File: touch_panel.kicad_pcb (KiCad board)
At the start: 2 copper layers, 50.5 x 50.5 mm, 52 parts, among them J1 2x4 SMD 2.0 MM, J2 2x4 Regular, Q1 MMBT2222, Q2 MMBT2222, Q3 MMBT2222, Q4 MMBT2222, Q5 MMBT2222, Q6 MMBT2222, SW1 Reset Switch, U1 TTP223_1, U2 TTP223_2, U3 TTP223_3, U4 ESP-12E

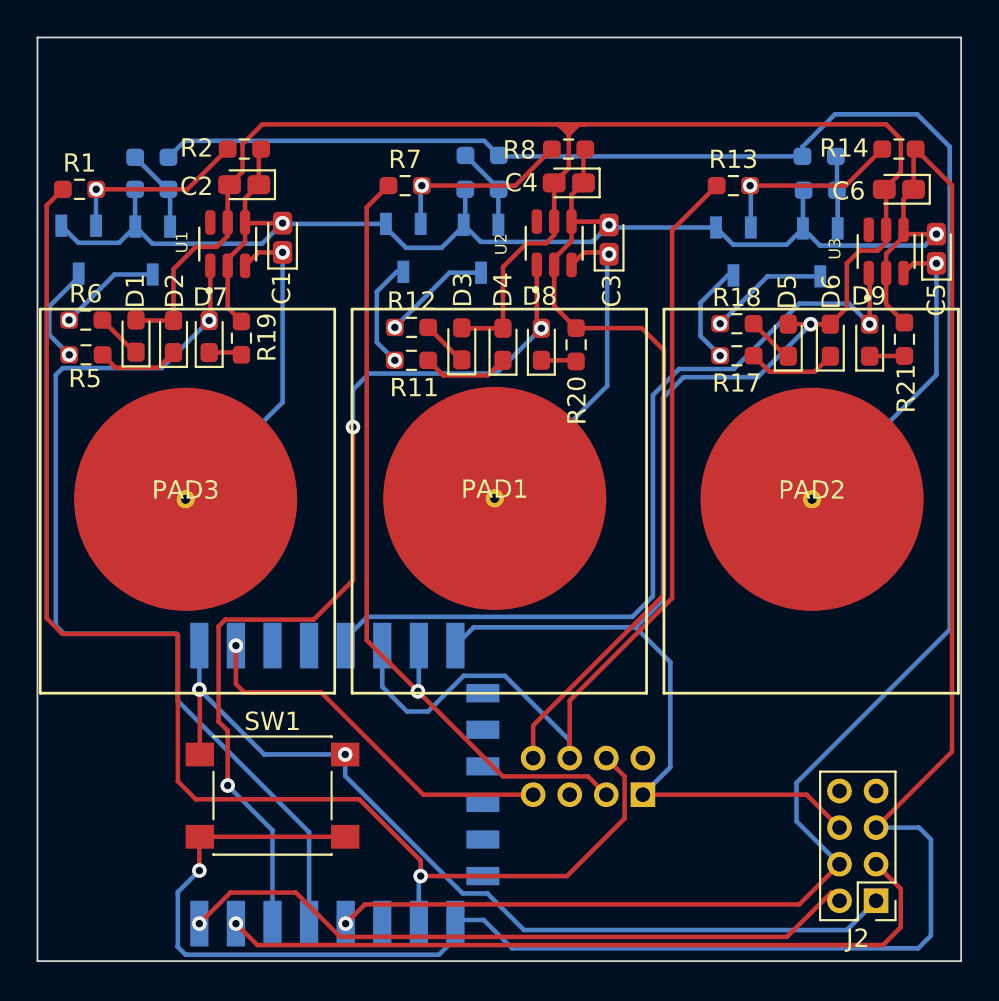
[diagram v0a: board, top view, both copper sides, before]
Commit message: Some changes performed
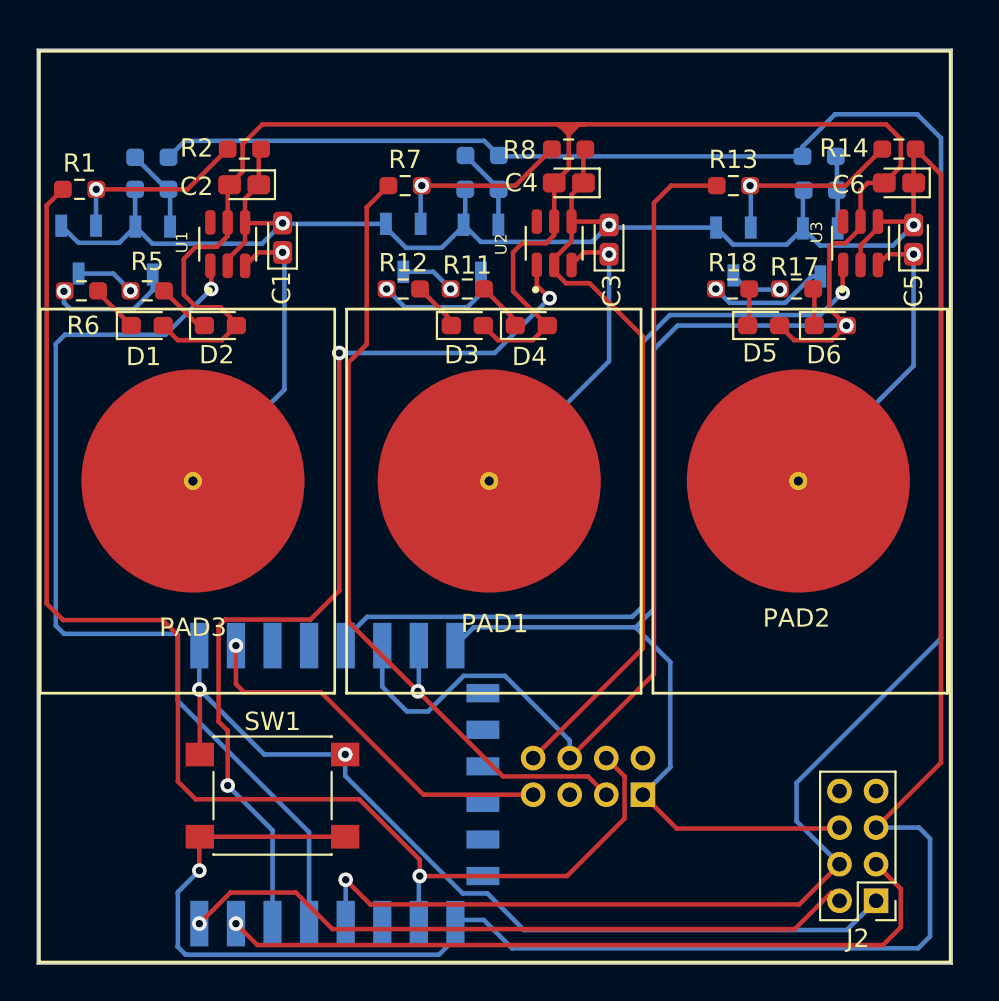
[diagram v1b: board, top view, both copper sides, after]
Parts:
- removed D7, D8, D9: RED, LED_SMD:LED_0603_1608Metric_Pad1.05x0.95mm_HandSolder
- removed R19, R20, R21: 1K, Resistor_SMD:R_0603_1608Metric_Pad0.98x0.95mm_HandSolder
- moved R11 4.95 mm to (131.0, 92.5)
- moved R17 4.90 mm to (149.0, 92.5)
- moved R5 4.84 mm to (113.5, 92.6)
- moved D2 2.63 mm to (117.5, 94.5), turned to 0 degrees
- moved R12 2.15 mm to (127.5, 92.5)
- moved R18 1.91 mm to (145.5, 92.5)
- moved D4 1.86 mm to (134.5, 94.5), turned to 0 degrees
- moved R6 1.62 mm to (109.9, 92.6)
- moved D5 1.57 mm to (147.2, 94.5), turned to 0 degrees
- moved U3 1.47 mm to (152.5, 90.0)
- moved C5 1.35 mm to (155.4, 89.8)
- moved PAD2 1.25 mm to (149.1, 103.0)
- moved PAD3 1.08 mm to (116.0, 103.0)
- moved D3 1.04 mm to (131.0, 94.5), turned to 0 degrees
- moved PAD1 1.00 mm to (132.2, 103.0)
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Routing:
- net +3V3: track 138.7 -> 152.3 mm
- net GND: track 234.3 -> 223.3 mm
- net Net-(Q3-Pad3): track 6.06 -> 2.98 mm
- net Net-(Q5-Pad3): track 5.76 -> 2.86 mm
- net Net-(D6-Pad1): track 4.91 -> 2.03 mm
- net Net-(Q1-Pad3): track 5.55 -> 3.42 mm
- net Net-(D4-Pad1): track 4.77 -> 2.71 mm
- net Net-(D9-Pad1): track 1.94 -> 0.00 mm
- net Net-(D8-Pad1): track 1.93 -> 0.00 mm
- net Net-(D7-Pad1): track 1.81 -> 0.00 mm
- net Net-(D2-Pad1): track 4.51 -> 3.00 mm
- net Relay 3: track 50.9 -> 52.4 mm
- net Net-(Q2-Pad3): track 5.61 -> 6.90 mm
- net Touch 2: track 51.6 -> 52.7 mm
- net Net-(C1-Pad1): track 18.0 -> 17.0 mm
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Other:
- board size 50.5 x 50.5 mm -> 50 x 50 mm
